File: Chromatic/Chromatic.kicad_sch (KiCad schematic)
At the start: 199 parts

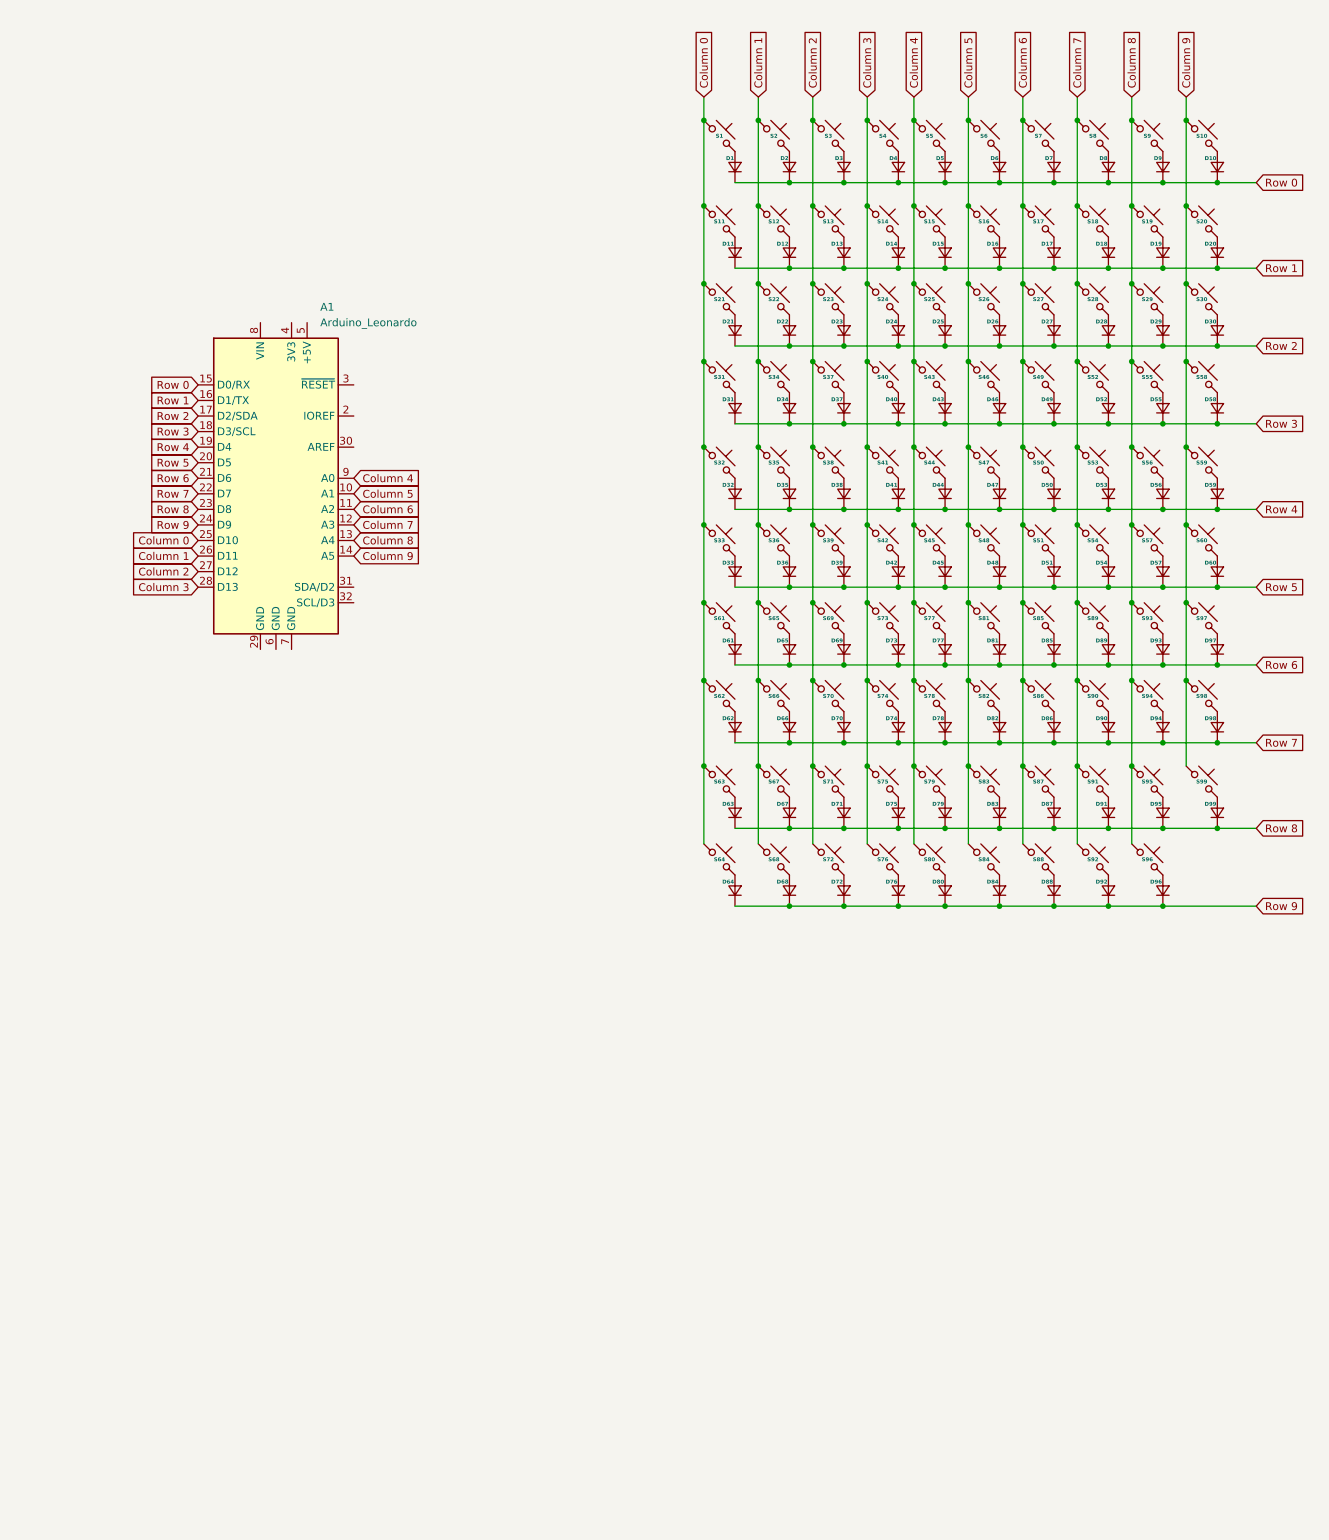
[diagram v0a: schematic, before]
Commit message: ATA
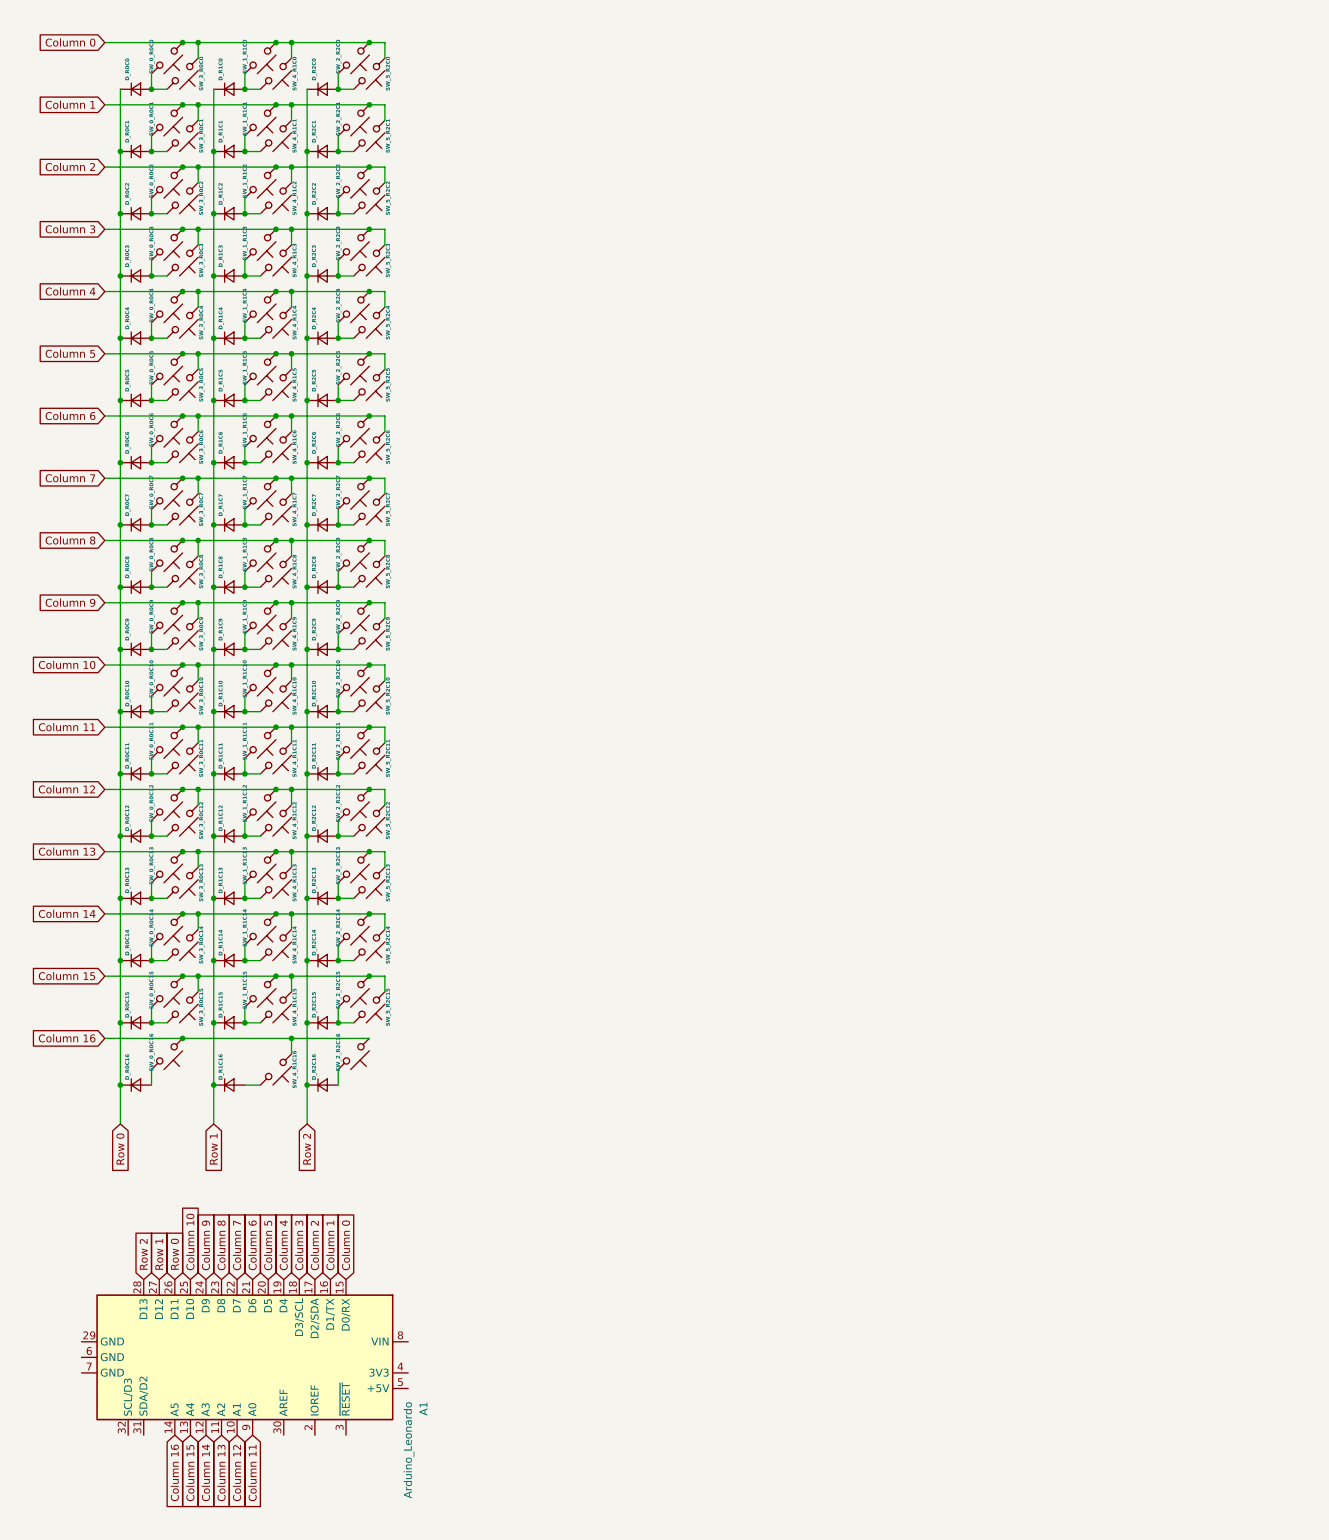
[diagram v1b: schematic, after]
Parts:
- removed D1, D10, D11, D12, D13, D14, D15, D16, D17, D18, D19, D2, D20, D21, D22, D23, D24, D25, D26, D27, D28, D29, D3, D30, D31, D32, D33, D34, D35, D36, D37, D38, D39, D4, D40, D41, D42, D43, D44, D45, D46, D47, D48, D49, D5, D50, D51, D52, D53, D54, D55, D56, D57, D58, D59, D6, D60, D61, D62, D63, D64, D65, D66, D67, D68, D69, D7, D70, D71, D72, D73, D74, D75, D76, D77, D78, D79, D8, D80, D81, D82, D83, D84, D85, D86, D87, D88, D89, D9, D90, D91, D92, D93, D94, D95, D96, D97, D98, D99: Diode, ScottoKeebs_Components:Diode_DO-35, symbol ScottoKeebs:Placeholder_Diode
- removed S1, S10, S11, S12, S13, S14, S15, S16, S17, S18, S19, S2, S20, S21, S22, S23, S24, S25, S26, S27, S28, S29, S3, S30, S31, S32, S33, S34, S35, S36, S37, S38, S39, S4, S40, S41, S42, S43, S44, S45, S46, S47, S48, S49, S5, S50, S51, S52, S53, S54, S55, S56, S57, S58, S59, S6, S60, S61, S62, S63, S64, S65, S66, S67, S68, S69, S7, S70, S71, S72, S73, S74, S75, S76, S77, S78, S79, S8, S80, S81, S82, S83, S84, S85, S86, S87, S88, S89, S9, S90, S91, S92, S93, S94, S95, S96, S97, S98, S99: Keyswitch, ScottoKeebs_MX:MX_PCB_1.00u, symbol ScottoKeebs:Placeholder_Keyswitch
- added D_R0C0, D_R0C1, D_R0C10, D_R0C11, D_R0C12, D_R0C13, D_R0C14, D_R0C15, D_R0C16, D_R0C2, D_R0C3, D_R0C4, D_R0C5, D_R0C6, D_R0C7, D_R0C8, D_R0C9, D_R1C0, D_R1C1, D_R1C10, D_R1C11, D_R1C12, D_R1C13, D_R1C14, D_R1C15, D_R1C16, D_R1C2, D_R1C3, D_R1C4, D_R1C5, D_R1C6, D_R1C7, D_R1C8, D_R1C9, D_R2C0, D_R2C1, D_R2C10, D_R2C11, D_R2C12, D_R2C13, D_R2C14, D_R2C15, D_R2C16, D_R2C2, D_R2C3, D_R2C4, D_R2C5, D_R2C6, D_R2C7, D_R2C8, D_R2C9: ~, ScottoKeebs_Components:Diode_DO-35, symbol ScottoKeebs:Placeholder_Diode
- added SW_0_R0C0, SW_0_R0C1, SW_0_R0C10, SW_0_R0C11, SW_0_R0C12, SW_0_R0C13, SW_0_R0C14, SW_0_R0C15, SW_0_R0C16, SW_0_R0C2, SW_0_R0C3, SW_0_R0C4, SW_0_R0C5, SW_0_R0C6, SW_0_R0C7, SW_0_R0C8, SW_0_R0C9, SW_1_R1C0, SW_1_R1C1, SW_1_R1C10, SW_1_R1C11, SW_1_R1C12, SW_1_R1C13, SW_1_R1C14, SW_1_R1C15, SW_1_R1C2, SW_1_R1C3, SW_1_R1C4, SW_1_R1C5, SW_1_R1C6, SW_1_R1C7, SW_1_R1C8, SW_1_R1C9, SW_2_R2C0, SW_2_R2C1, SW_2_R2C10, SW_2_R2C11, SW_2_R2C12, SW_2_R2C13, SW_2_R2C14, SW_2_R2C15, SW_2_R2C16, SW_2_R2C2, SW_2_R2C3, SW_2_R2C4, SW_2_R2C5, SW_2_R2C6, SW_2_R2C7, SW_2_R2C8, SW_2_R2C9, SW_3_R0C0, SW_3_R0C1, SW_3_R0C10, SW_3_R0C11, SW_3_R0C12, SW_3_R0C13, SW_3_R0C14, SW_3_R0C15, SW_3_R0C2, SW_3_R0C3, SW_3_R0C4, SW_3_R0C5, SW_3_R0C6, SW_3_R0C7, SW_3_R0C8, SW_3_R0C9, SW_4_R1C0, SW_4_R1C1, SW_4_R1C10, SW_4_R1C11, SW_4_R1C12, SW_4_R1C13, SW_4_R1C14, SW_4_R1C15, SW_4_R1C16, SW_4_R1C2, SW_4_R1C3, SW_4_R1C4, SW_4_R1C5, SW_4_R1C6, SW_4_R1C7, SW_4_R1C8, SW_4_R1C9, SW_5_R2C0, SW_5_R2C1, SW_5_R2C10, SW_5_R2C11, SW_5_R2C12, SW_5_R2C13, SW_5_R2C14, SW_5_R2C15, SW_5_R2C2, SW_5_R2C3, SW_5_R2C4, SW_5_R2C5, SW_5_R2C6, SW_5_R2C7, SW_5_R2C8, SW_5_R2C9: Keyswitch, ScottoKeebs_Hotswap:Hotswap_MX_1.00u, symbol ScottoKeebs:Placeholder_Keyswitch
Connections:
- net Row 3 is gone; now on net Column 3: A1.18 (D3/SCL)
- net Row 4 is gone; now on net Column 4: A1.19 (D4)
- net Row 5 is gone; now on net Column 5: A1.20 (D5)
- net Row 6 is gone; now on net Column 6: A1.21 (D6)
- net Row 7 is gone; now on net Column 7: A1.22 (D7)
- net Row 8 is gone; now on net Column 8: A1.23 (D8)
- net Row 9 is gone; now on net Column 9: A1.24 (D9)
- net Column 0: now also A1.15 (D0/RX), SW_0_R0C0.1, SW_1_R1C0.1, SW_2_R2C0.1, SW_3_R0C0.1, SW_4_R1C0.1, SW_5_R2C0.1; no longer A1.25 (D10)
- net Column 1: now also A1.16 (D1/TX), SW_0_R0C1.1, SW_1_R1C1.1, SW_2_R2C1.1, SW_3_R0C1.1, SW_4_R1C1.1, SW_5_R2C1.1; no longer A1.26 (D11)
- net Column 2: now also A1.17 (D2/SDA), SW_0_R0C2.1, SW_1_R1C2.1, SW_2_R2C2.1, SW_3_R0C2.1, SW_4_R1C2.1, SW_5_R2C2.1; no longer A1.27 (D12)
- net Column 3: now also SW_0_R0C3.1, SW_1_R1C3.1, SW_2_R2C3.1, SW_3_R0C3.1, SW_4_R1C3.1, SW_5_R2C3.1; no longer A1.28 (D13)
- net Column 4: now also SW_0_R0C4.1, SW_1_R1C4.1, SW_2_R2C4.1, SW_3_R0C4.1, SW_4_R1C4.1, SW_5_R2C4.1; no longer A1.9 (A0)
- net Column 5: now also SW_0_R0C5.1, SW_1_R1C5.1, SW_2_R2C5.1, SW_3_R0C5.1, SW_4_R1C5.1, SW_5_R2C5.1; no longer A1.10 (A1)
- net Column 6: now also SW_0_R0C6.1, SW_1_R1C6.1, SW_2_R2C6.1, SW_3_R0C6.1, SW_4_R1C6.1, SW_5_R2C6.1; no longer A1.11 (A2)
- net Column 7: now also SW_0_R0C7.1, SW_1_R1C7.1, SW_2_R2C7.1, SW_3_R0C7.1, SW_4_R1C7.1, SW_5_R2C7.1; no longer A1.12 (A3)
- net Column 8: now also SW_0_R0C8.1, SW_1_R1C8.1, SW_2_R2C8.1, SW_3_R0C8.1, SW_4_R1C8.1, SW_5_R2C8.1; no longer A1.13 (A4)
- net Column 9: now also SW_0_R0C9.1, SW_1_R1C9.1, SW_2_R2C9.1, SW_3_R0C9.1, SW_4_R1C9.1, SW_5_R2C9.1; no longer A1.14 (A5)
- net Row 0: now also A1.26 (D11), D_R0C0.1 (K), D_R0C1.1 (K), D_R0C10.1 (K), D_R0C11.1 (K), D_R0C12.1 (K), D_R0C13.1 (K), D_R0C14.1 (K), D_R0C15.1 (K), D_R0C16.1 (K), D_R0C2.1 (K), D_R0C3.1 (K), D_R0C4.1 (K), D_R0C5.1 (K), D_R0C6.1 (K), D_R0C7.1 (K), D_R0C8.1 (K), D_R0C9.1 (K); no longer A1.15 (D0/RX)
- net Row 1: now also A1.27 (D12), D_R1C0.1 (K), D_R1C1.1 (K), D_R1C10.1 (K), D_R1C11.1 (K), D_R1C12.1 (K), D_R1C13.1 (K), D_R1C14.1 (K), D_R1C15.1 (K), D_R1C16.1 (K), D_R1C2.1 (K), D_R1C3.1 (K), D_R1C4.1 (K), D_R1C5.1 (K), D_R1C6.1 (K), D_R1C7.1 (K), D_R1C8.1 (K), D_R1C9.1 (K); no longer A1.16 (D1/TX)
- net Row 2: now also A1.28 (D13), D_R2C0.1 (K), D_R2C1.1 (K), D_R2C10.1 (K), D_R2C11.1 (K), D_R2C12.1 (K), D_R2C13.1 (K), D_R2C14.1 (K), D_R2C15.1 (K), D_R2C16.1 (K), D_R2C2.1 (K), D_R2C3.1 (K), D_R2C4.1 (K), D_R2C5.1 (K), D_R2C6.1 (K), D_R2C7.1 (K), D_R2C8.1 (K), D_R2C9.1 (K); no longer A1.17 (D2/SDA)
- new net: D_R1C7.2 (A), SW_1_R1C7.2, SW_4_R1C7.2
- new net: D_R0C3.2 (A), SW_0_R0C3.2, SW_3_R0C3.2
- new net: D_R2C4.2 (A), SW_2_R2C4.2, SW_5_R2C4.2
- new net: D_R0C16.2 (A), SW_0_R0C16.2
- new net: D_R1C0.2 (A), SW_1_R1C0.2, SW_4_R1C0.2
- new net: D_R2C2.2 (A), SW_2_R2C2.2, SW_5_R2C2.2
- new net: D_R0C1.2 (A), SW_0_R0C1.2, SW_3_R0C1.2
- new net: D_R1C8.2 (A), SW_1_R1C8.2, SW_4_R1C8.2
- new net: D_R1C13.2 (A), SW_1_R1C13.2, SW_4_R1C13.2
- new net: D_R2C1.2 (A), SW_2_R2C1.2, SW_5_R2C1.2
- new net: D_R2C6.2 (A), SW_2_R2C6.2, SW_5_R2C6.2
- new net: D_R2C5.2 (A), SW_2_R2C5.2, SW_5_R2C5.2
- new net: D_R1C3.2 (A), SW_1_R1C3.2, SW_4_R1C3.2
- new net: D_R0C15.2 (A), SW_0_R0C15.2, SW_3_R0C15.2
- new net: D_R1C15.2 (A), SW_1_R1C15.2, SW_4_R1C15.2
- new net: D_R2C0.2 (A), SW_2_R2C0.2, SW_5_R2C0.2
- new net: D_R1C4.2 (A), SW_1_R1C4.2, SW_4_R1C4.2
- new net: D_R2C13.2 (A), SW_2_R2C13.2, SW_5_R2C13.2
- new net: D_R0C14.2 (A), SW_0_R0C14.2, SW_3_R0C14.2
- new net: D_R0C7.2 (A), SW_0_R0C7.2, SW_3_R0C7.2
- new net: D_R0C0.2 (A), SW_0_R0C0.2, SW_3_R0C0.2
- new net: D_R1C9.2 (A), SW_1_R1C9.2, SW_4_R1C9.2
- new net: D_R1C1.2 (A), SW_1_R1C1.2, SW_4_R1C1.2
- new net: D_R0C2.2 (A), SW_0_R0C2.2, SW_3_R0C2.2
- new net: D_R1C6.2 (A), SW_1_R1C6.2, SW_4_R1C6.2
- new net: D_R0C13.2 (A), SW_0_R0C13.2, SW_3_R0C13.2
- new net: D_R2C16.2 (A), SW_2_R2C16.2
- new net: D_R0C6.2 (A), SW_0_R0C6.2, SW_3_R0C6.2
- new net: D_R2C15.2 (A), SW_2_R2C15.2, SW_5_R2C15.2
- new net: D_R0C11.2 (A), SW_0_R0C11.2, SW_3_R0C11.2
- new net: D_R1C11.2 (A), SW_1_R1C11.2, SW_4_R1C11.2
- new net: D_R1C2.2 (A), SW_1_R1C2.2, SW_4_R1C2.2
- new net: D_R2C9.2 (A), SW_2_R2C9.2, SW_5_R2C9.2
- new net: D_R2C10.2 (A), SW_2_R2C10.2, SW_5_R2C10.2
- new net: D_R2C3.2 (A), SW_2_R2C3.2, SW_5_R2C3.2
- new net: D_R1C5.2 (A), SW_1_R1C5.2, SW_4_R1C5.2
- new net: D_R0C8.2 (A), SW_0_R0C8.2, SW_3_R0C8.2
- new net: D_R1C16.2 (A), SW_4_R1C16.2
- new net: D_R2C8.2 (A), SW_2_R2C8.2, SW_5_R2C8.2
- new net: D_R0C5.2 (A), SW_0_R0C5.2, SW_3_R0C5.2
- new net: D_R0C4.2 (A), SW_0_R0C4.2, SW_3_R0C4.2
- new net: D_R2C12.2 (A), SW_2_R2C12.2, SW_5_R2C12.2
- new net: D_R2C7.2 (A), SW_2_R2C7.2, SW_5_R2C7.2
- new net: D_R0C9.2 (A), SW_0_R0C9.2, SW_3_R0C9.2
- new net: D_R0C10.2 (A), SW_0_R0C10.2, SW_3_R0C10.2
- new net: D_R2C14.2 (A), SW_2_R2C14.2, SW_5_R2C14.2
- new net: D_R2C11.2 (A), SW_2_R2C11.2, SW_5_R2C11.2
- new net: D_R1C14.2 (A), SW_1_R1C14.2, SW_4_R1C14.2
- new net: D_R1C10.2 (A), SW_1_R1C10.2, SW_4_R1C10.2
- new net: D_R1C12.2 (A), SW_1_R1C12.2, SW_4_R1C12.2
- new net: D_R0C12.2 (A), SW_0_R0C12.2, SW_3_R0C12.2
- new net Column 10: A1.25 (D10), SW_0_R0C10.1, SW_1_R1C10.1, SW_2_R2C10.1, SW_3_R0C10.1, SW_4_R1C10.1, SW_5_R2C10.1
- new net Column 11: A1.9 (A0), SW_0_R0C11.1, SW_1_R1C11.1, SW_2_R2C11.1, SW_3_R0C11.1, SW_4_R1C11.1, SW_5_R2C11.1
- new net Column 12: A1.10 (A1), SW_0_R0C12.1, SW_1_R1C12.1, SW_2_R2C12.1, SW_3_R0C12.1, SW_4_R1C12.1, SW_5_R2C12.1
- new net Column 13: A1.11 (A2), SW_0_R0C13.1, SW_1_R1C13.1, SW_2_R2C13.1, SW_3_R0C13.1, SW_4_R1C13.1, SW_5_R2C13.1
- new net Column 14: A1.12 (A3), SW_0_R0C14.1, SW_1_R1C14.1, SW_2_R2C14.1, SW_3_R0C14.1, SW_4_R1C14.1, SW_5_R2C14.1
- new net Column 15: A1.13 (A4), SW_0_R0C15.1, SW_1_R1C15.1, SW_2_R2C15.1, SW_3_R0C15.1, SW_4_R1C15.1, SW_5_R2C15.1
- new net Column 16: A1.14 (A5), SW_0_R0C16.1, SW_2_R2C16.1, SW_4_R1C16.1
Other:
- moved on the sheet: A1
